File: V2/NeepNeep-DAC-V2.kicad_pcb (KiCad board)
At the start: 2 copper layers, 24 x 24 mm, 17 parts, among them J1 Conn_02x03_Odd_Even, J2 Conn_01x03_Pin, Q1 BSS138, U2 W25Q32JVSS, U3 ATtiny85-20SU

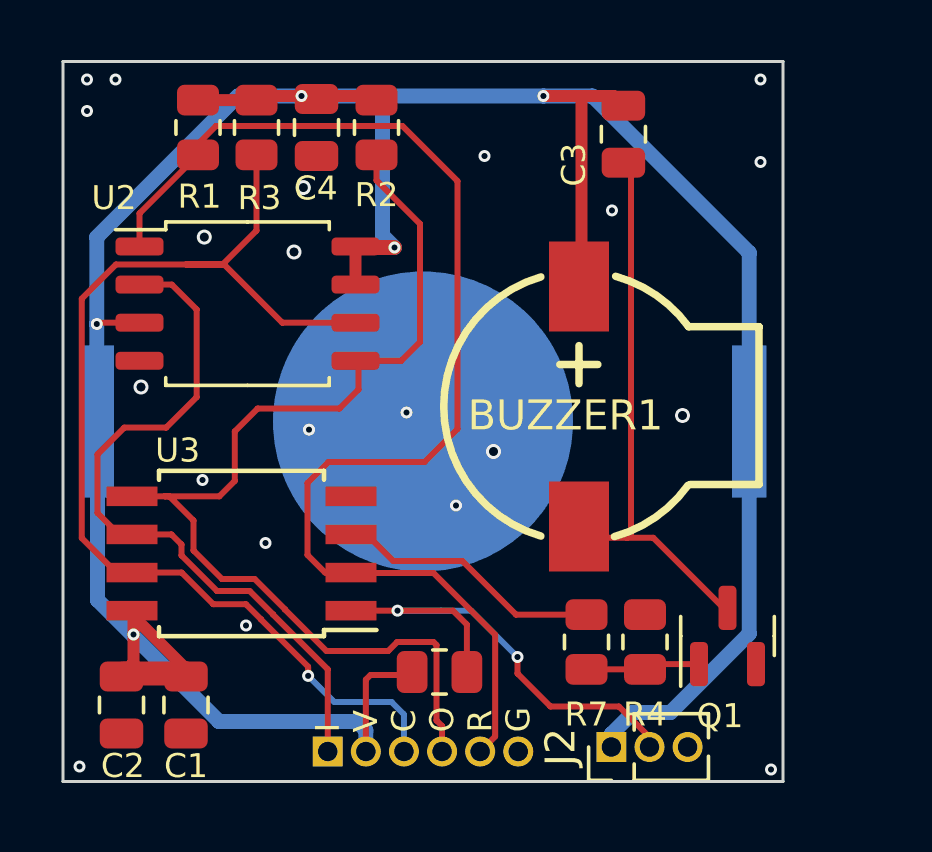
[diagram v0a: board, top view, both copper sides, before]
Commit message: Commit: M	README.md A	V2/NeepNeep-DAC-V2-backups/NeepNeep-DAC-V2-2026-02-12_124743.zip A	V2/NeepNeep-DAC-V2-backups/NeepNeep-DAC-V2-2026-02-12_132550.zip A	V2/NeepNeep-DAC-V2-backups/NeepNeep-DAC-V2-2026-02-12_133556.zip A	V2/NeepNeep-DAC-V2-backups/NeepNeep-DAC-V2-2026-02-12_142149.zip A	V2/NeepNeep-DAC-V2-backups/NeepNeep-DAC-V2-2026-02-12_143905.zip A	V2/NeepNeep-DAC-V2-backups/NeepNeep-DAC-V2-2026-02-12_170144.zip M	V2/NeepNeep-DAC-V2.kicad_pcb M	V2/NeepNeep-DAC-V2.kicad_prl M	V2/NeepNeep-DAC-V2.kicad_pro M	V2/NeepNeep-DAC-V2.kicad_sch A	V2/bom/NeepNeep-DAC-V2-ibom.html M	V2/fp-info-cache A	V2/ibom.config.ini A	V2/jlcpcb/gerber/NeepNeep-DAC-V2-CuBottom.gbr A	V2/jlcpcb/gerber/NeepNeep-DAC-V2-CuTop.gbr A	V2/jlcpcb/gerber/NeepNeep-DAC-V2-EdgeCuts.gbr A	V2/jlcpcb/gerber/NeepNeep-DAC-V2-MaskBottom.gbr A	V2/jlcpcb/gerber/NeepNeep-DAC-V2-MaskTop.gbr A	V2/jlcpcb/gerber/NeepNeep-DAC-V2-NPTH-drl_map.pdf A	V2/jlcpcb/gerber/NeepNeep-DAC-V2-NPTH.drl A	V2/jlcpcb/gerber/NeepNeep-DAC-V2-PTH-drl_map.pdf A	V2/jlcpcb/gerber/NeepNeep-DAC-V2-PTH.drl A	V2/jlcpcb/gerber/NeepNeep-DAC-V2-PasteBottom.gbr A	V2/jlcpcb/gerber/NeepNeep-DAC-V2-PasteTop.gbr A	V2/jlcpcb/gerber/NeepNeep-DAC-V2-SilkBottom.gbr A	V2/jlcpcb/gerber/NeepNeep-DAC-V2-SilkTop.gbr A	V2/jlcpcb/gerber/NeepNeep-DAC-V2-VScore.gbr A	V2/jlcpcb/production_files/BOM-NeepNeep-DAC-V2.csv A	V2/jlcpcb/production_files/CPL-NeepNeep-DAC-V2.csv A	V2/jlcpcb/production_files/GERBER-NeepNeep-DAC-V2.zip A	V2/jlcpcb/project.db
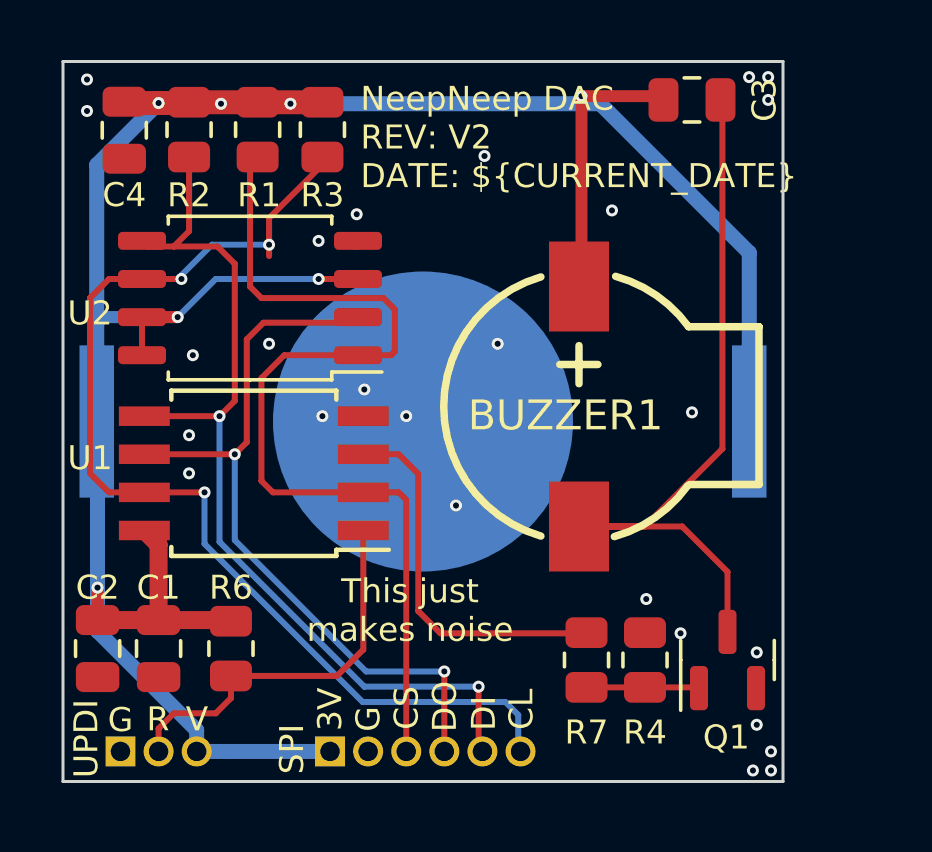
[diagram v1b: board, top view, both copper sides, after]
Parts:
- J1: footprint Global Kicad FootprintLibrary:PRG-Header_1x06_P1.27mm -> Niffum-Connector:SPI-Header_1x06_P1.27mm
- J2: footprint Connector_PinHeader_1.27mm:PinHeader_1x03_P1.27mm_Vertical -> Niffum-Connector:UPDI PinHeader_1x03_P1.27mm_Vertical
- moved J2 16.4 mm to (89.9, 111.0)
- moved R6 6.99 mm to (93.6, 107.6), turned to -90 degrees
- moved C4 6.41 mm to (90.0, 90.3)
- moved R2 6.25 mm to (92.2, 90.3)
- moved U1 2.70 mm to (94.4, 101.7)
- moved C3 2.56 mm to (109.0, 89.3), turned to 0 degrees
- moved R3 2.20 mm to (96.6, 90.3)
- moved C1 2.09 mm to (91.2, 107.6)
- moved C2 2.04 mm to (89.2, 107.6)
- moved R1 1.99 mm to (94.5, 90.3)
- moved Q1 0.80 mm to (110.2, 108.0)
- moved R4 0.60 mm to (107.4, 108.0)
- moved R7 0.60 mm to (105.5, 108.0)
- moved U2 0.20 mm to (94.2, 95.9), turned to 180 degrees
- moved J1 0.08 mm to (96.9, 111.0)
- renumbered U3 to U1
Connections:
- J1 pad 1: PB1/MISO -> 3.3v
- J1 pad 2: 3.3v -> GND
- J1 pad 3: PB2/SCK -> PB3
- J1 pad 4: PB0/MOSI -> PB1/MISO
- J1 pad 5: PB3 -> PB0/MOSI
- J1 pad 6: GND -> PB2/SCK
- J2 pad 1: 3.3v -> GND
- J2 pad 3: GND -> 3.3v
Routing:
- net 3.3v: track 104.3 -> 92.9 mm, vias 5 -> 7
- net PB3: track 42.6 -> 32.7 mm
- net Net-(BUZZER1--): track 18.8 -> 25.1 mm
- net PB0/MOSI: track 35.8 -> 31.7 mm, vias 0 -> 2
- net PB4: track 8.96 -> 12.6 mm
- net PB5/RESET: track 16.4 -> 13.1 mm, vias 2 -> 0
- net PB2/SCK: track 38.3 -> 36.5 mm, vias 1 -> 3
- net PB1/MISO: track 24.0 -> 25.4 mm, vias 0 -> 2
- net GND: track 0.00 -> 0.07 mm, vias 21 -> 26
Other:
- board text added: "${TITLE} REV: ${REVISION} DATE: ${CURRENT_DATE}"
- board text added: "SPI"
- board text added: "UPDI"
- board text removed: "${TITLE} REV: ${REVISION}"
- board text removed: "DATE: ${CURRENT_DATE}"
